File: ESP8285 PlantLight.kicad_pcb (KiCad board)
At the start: 2 copper layers, 55 parts, among them J1 Conn_01x03_Female, Q1 P-Chan Mosfet, Q2 Q_NPN_BCE, Q3 Q_PNP_BCE, U1 ESP8285, U3 SFH617A-1X007T, U4 SFH617A-1X007T, Y1 26Mhz

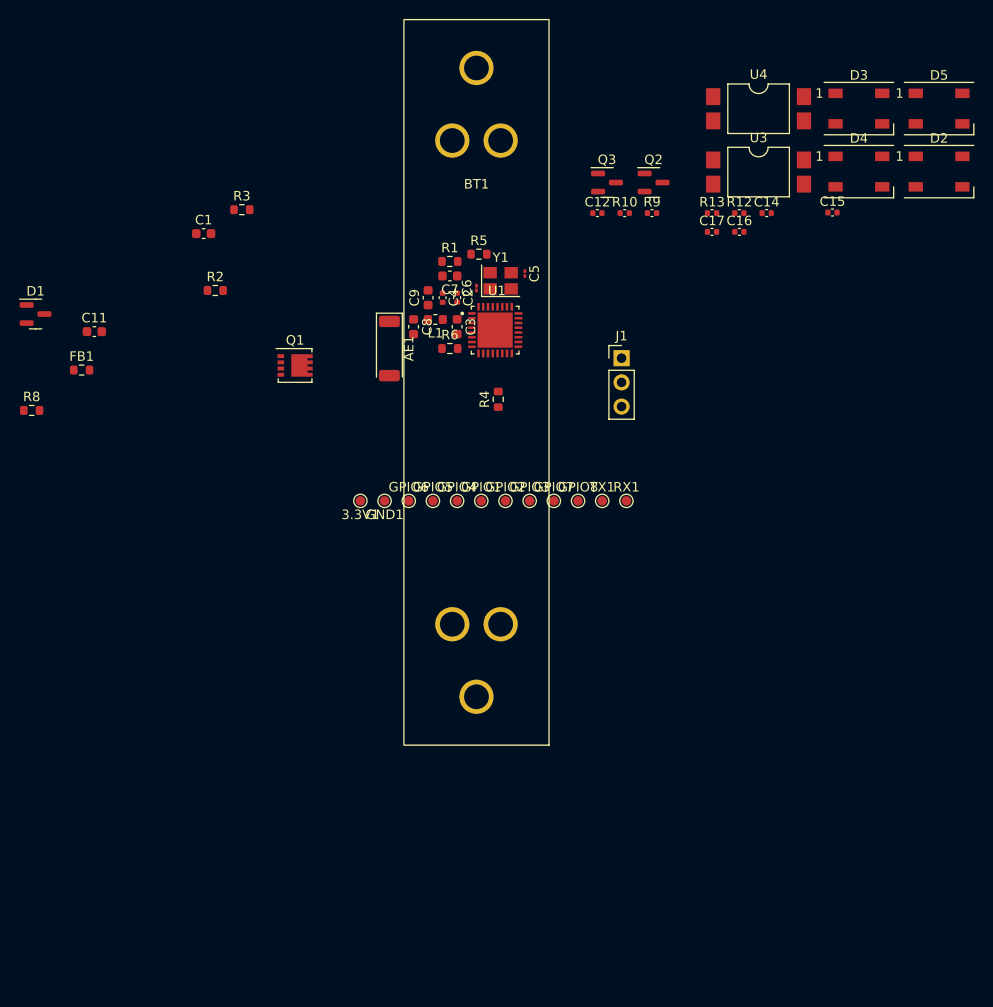
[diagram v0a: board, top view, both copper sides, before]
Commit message: mon
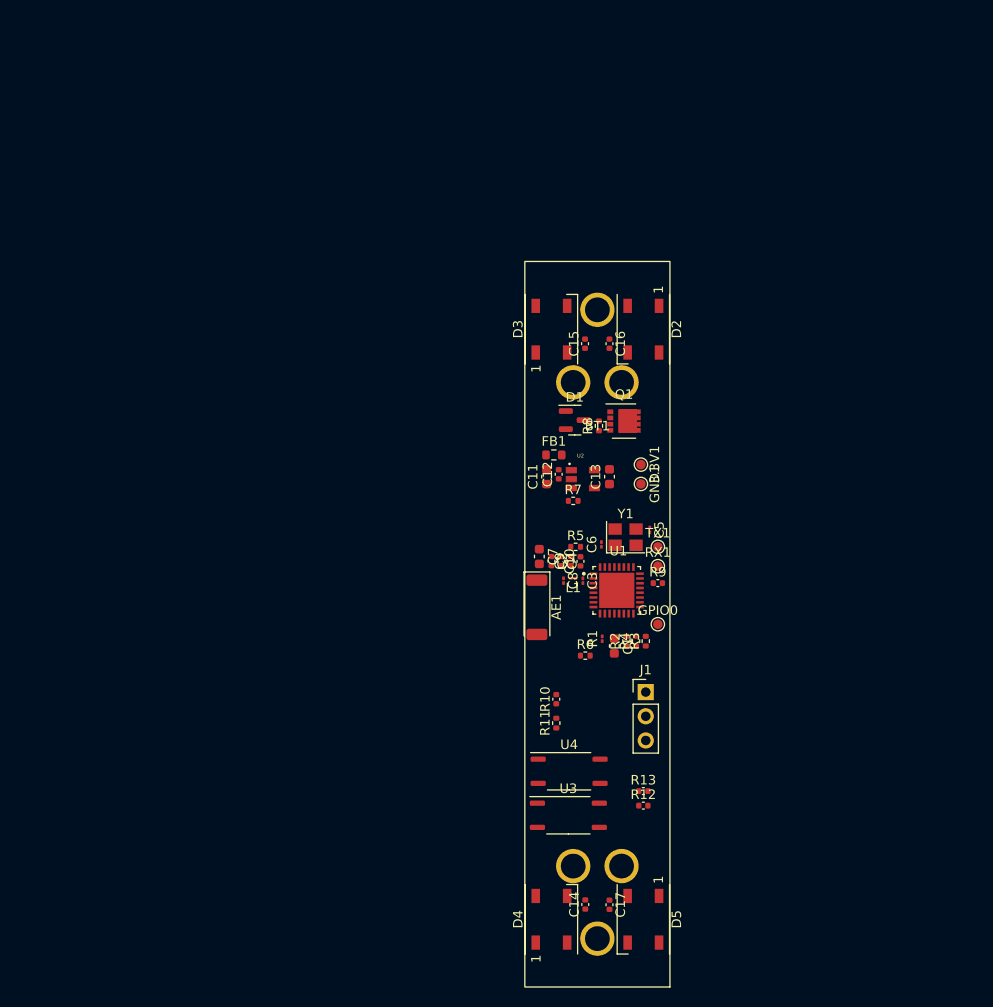
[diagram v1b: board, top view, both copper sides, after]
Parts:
- removed GPIO1, GPIO2, GPIO3, GPIO4, GPIO5, GPIO6, GPIO7, GPIO8: TestPoint_Small, TestPoint:TestPoint_Pad_D1.0mm
- removed Q2: Q_NPN_BCE, Package_TO_SOT_SMD:SOT-23
- removed Q3: Q_PNP_BCE, Package_TO_SOT_SMD:SOT-23
- added C10: 100nF, Capacitor_SMD:C_0402_1005Metric, F.Cu at (150.6, 72.1)
- added C13: 1uF, Capacitor_SMD:C_0603_1608Metric, F.Cu at (153.7, 63.2)
- added GPIO0: TestPoint_Small, TestPoint:TestPoint_Pad_D1.0mm, F.Cu at (158.8, 78.7)
- added R11: 300K, Resistor_SMD:R_0402_1005Metric, F.Cu at (148.1, 89.1)
- added R7: 10K, Resistor_SMD:R_0402_1005Metric, F.Cu at (149.9, 65.8)
- added U2: RT9193-33GB, RT9193-33GB:SOT94P279X129-5N, F.Cu at (150.9, 63.5)
- C3, C8: footprint Capacitor_SMD:C_0603_1608Metric -> Capacitor_SMD:C_01005_0402Metric
- C9: footprint Capacitor_SMD:C_0603_1608Metric -> Capacitor_SMD:C_0402_1005Metric
- J1: value Conn_01x03_Female -> 01x03
- L1: footprint Inductor_SMD:L_0603_1608Metric -> Inductor_SMD:L_01005_0402Metric
- Q1: footprint Package_SON:Diodes_PowerDI3333-8 -> Package_SON:VSON-8_3.3x3.3mm_P0.65mm_NexFET
- R1: footprint Resistor_SMD:R_0603_1608Metric -> Resistor_SMD:R_01005_0402Metric
- R2, R3, R4, R5, R6, R8: footprint Resistor_SMD:R_0603_1608Metric -> Resistor_SMD:R_0402_1005Metric
- U3, U4: value SFH617A-1X007T -> TLP185; footprint Package_DIP:SMDIP-4_W9.53mm_Clearance8mm -> Package_SO:SOIC-4_4.55x3.7mm_P2.54mm
- moved D5 90.6 mm to (157.2, 109.7), turned to -90 degrees
- moved D4 84.9 mm to (147.6, 109.7), turned to 90 degrees
- moved C14 75.1 mm to (151.1, 108.2), turned to 90 degrees
- moved U4 72.4 mm to (149.4, 94.2)
- moved C17 71.5 mm to (153.7, 108.2), turned to -90 degrees
- moved U3 70.4 mm to (149.4, 98.8)
- moved R12 63.0 mm to (157.2, 97.8)
- moved R3 62.1 mm to (157.5, 80.5), turned to 90 degrees
- moved R13 61.1 mm to (157.2, 96.3)
- moved C1 61.1 mm to (154.2, 81.0), turned to -90 degrees
- moved R8 59.6 mm to (152.6, 57.9), turned to 90 degrees
- moved D1 57.7 mm to (150.0, 57.3)
- moved R2 56.8 mm to (155.4, 80.5), turned to 90 degrees
- moved R10 51.6 mm to (148.1, 86.6), turned to 90 degrees
- moved FB1 50.4 mm to (147.8, 61.0)
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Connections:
- net GPIO15 renamed /GPIO15
- net GPIO2 renamed /GPIO2
- 3.3V1 pad 1: VDD3V3 -> 3V3
- AE1 pad 2: (no net) -> unconnected-(AE1-Pad2)
- BT1 pad 1: +BATT -> /+BAT
- C14 pad 1: /V_BAT -> V_BAT
- C15 pad 1: /V_BAT -> V_BAT
- C16 pad 1: /V_BAT -> V_BAT
- C17 pad 1: /V_BAT -> V_BAT
- C2 pad 2: VDD3V3 -> 3V3
- C4 pad 2: VDD3V3 -> 3V3
- C7 pad 2: VDD3V3 -> 3V3
- C9 pad 1: VDD3V3 -> 3V3
- D1 pad 1: Net-(D1-Pad1) -> GND
- D1 pad 3: GND -> Net-(D1-Pad3)
- D2 pad 1: /V_BAT -> V_BAT
- D3 pad 1: /V_BAT -> V_BAT
- D4 pad 1: /V_BAT -> V_BAT
- D5 pad 1: /V_BAT -> V_BAT
- FB1 pad 1: /V_Bat -> V_BAT
- J1 pad 1: Net-(J1-Pad1) -> /J1_ADC_IN
- J1 pad 2: GND -> V_BAT
- J1 pad 3: +BATT -> GND
- Q1 pad 1: /V_Bat -> /+BAT
- Q1 pad 2: /V_Bat -> /+BAT
- Q1 pad 3: /V_Bat -> /+BAT
- Q1 pad 5: +BATT -> V_BAT
- R1 pad 1: +3V3 -> 3V3
- R10 pad 2: /V_BAT -> V_BAT
- R12 pad 1: /V_BAT -> V_BAT
- R3 pad 1: +3V3 -> 3V3
- R4 pad 1: +3V3 -> 3V3
- R6 pad 1: +3V3 -> 3V3
- R8 pad 2: Net-(D1-Pad1) -> Net-(D1-Pad3)
- U1 pad 1: VDD3V3 -> 3V3
- U1 pad 11: VDD3V3 -> 3V3
- U1 pad 17: VDD3V3 -> 3V3
- U1 pad 2: Net-(C3-Pad1) -> /LNA
- U1 pad 27: Net-(U1-Pad27) -> Net-(C5-Pad1)
- U1 pad 29: VDD3V3 -> 3V3
- U1 pad 3: VDD3V3 -> 3V3
- U1 pad 30: VDD3V3 -> 3V3
- U1 pad 4: VDD3V3 -> 3V3
- U3 pad 1: Net-(R9-Pad2) -> Net-(R12-Pad2)
- U3 pad 3: ADC -> Net-(R9-Pad2)
- U3 pad 4: Net-(J1-Pad1) -> ADC
- U4 pad 1: Net-(R12-Pad2) -> Net-(R9-Pad2)
- U4 pad 3: ADC -> Net-(R13-Pad1)
- U4 pad 4: Net-(R10-Pad1) -> ADC
